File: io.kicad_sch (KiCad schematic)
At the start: 1 part, among them U1 Allwinner_V3s

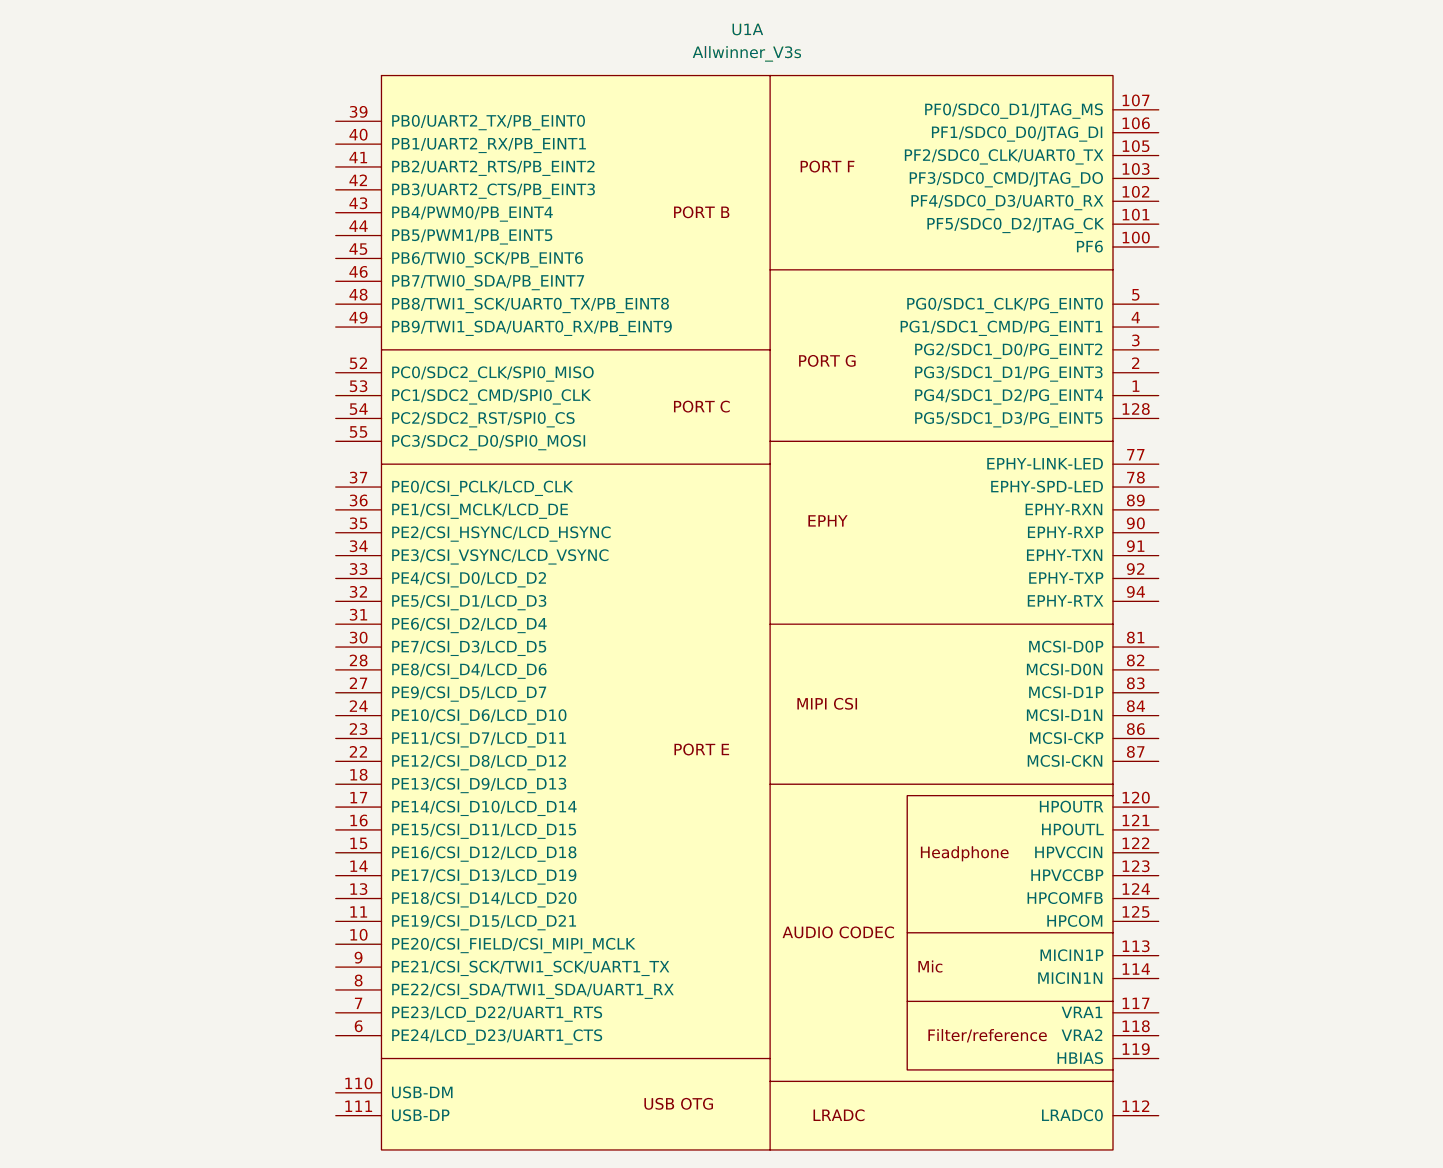
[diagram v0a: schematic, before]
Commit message: did some routing
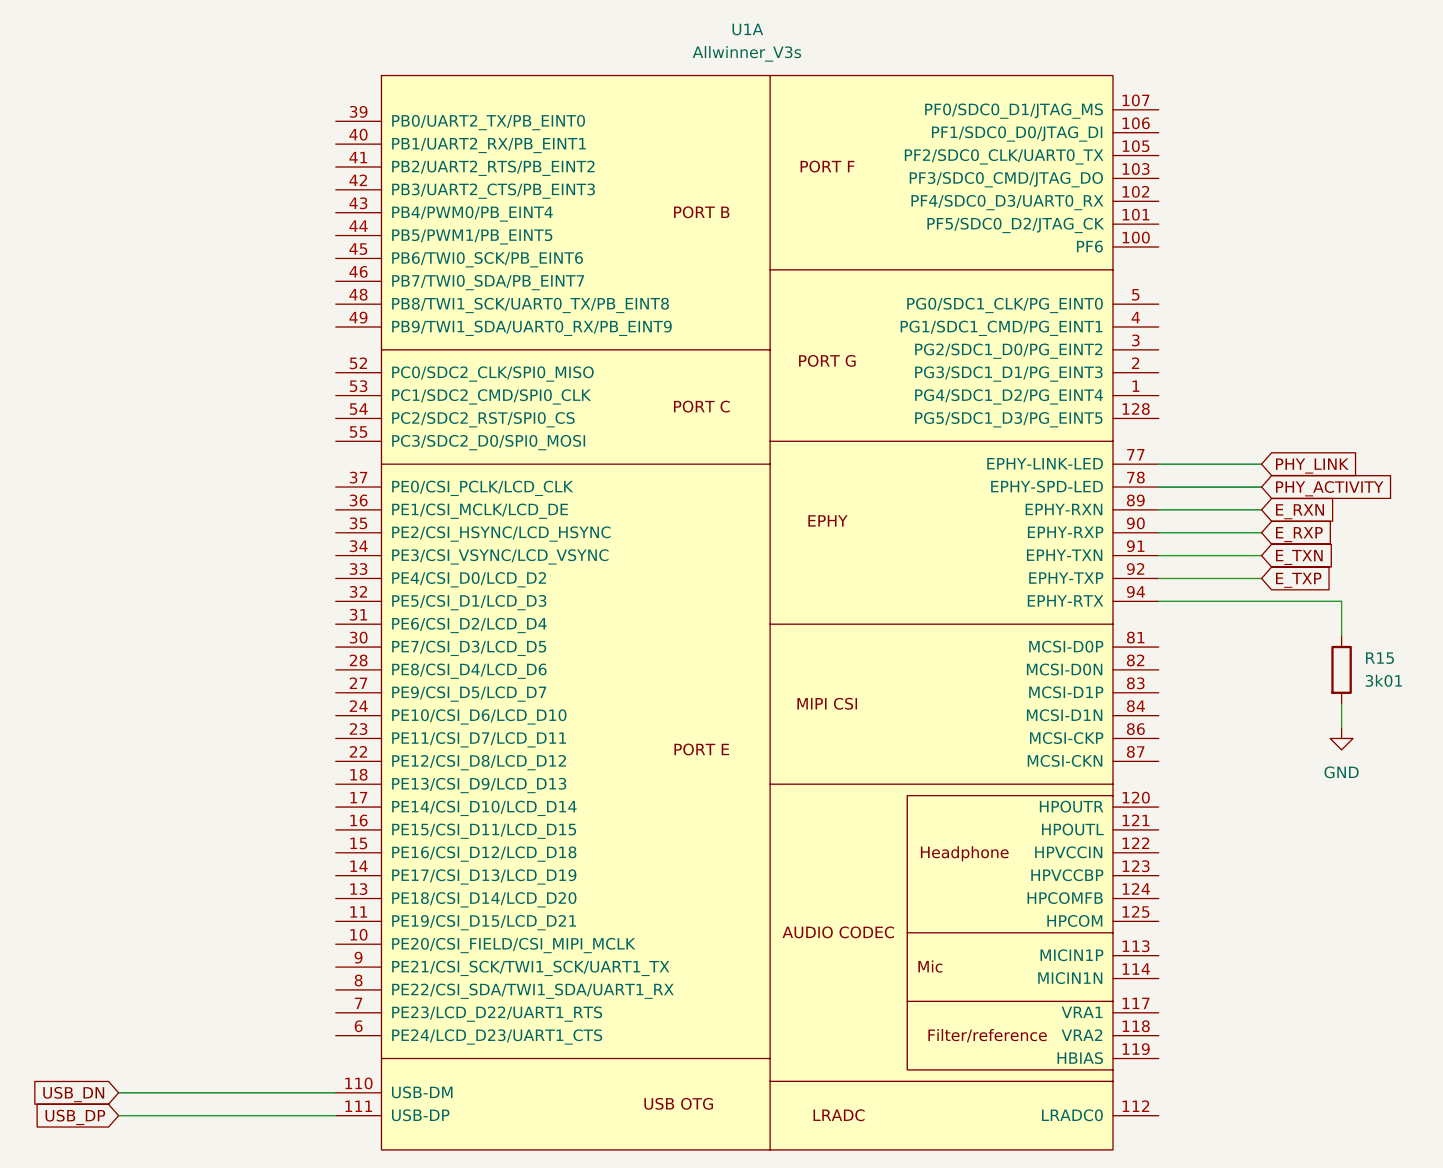
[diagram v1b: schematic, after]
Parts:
- added R15: 3k01, Resistor_SMD:R_0603_1608Metric, symbol Device:R
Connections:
- net USB_DN: now reaches U1.110 (USB-DM)
- net USB_DP: now reaches U1.111 (USB-DP)
- net PHY_LINK: now reaches U1.77 (EPHY-LINK-LED)
- net PHY_ACTIVITY: now reaches U1.78 (EPHY-SPD-LED)
- net E_RXN: now reaches U1.89 (EPHY-RXN)
- net E_RXP: now reaches U1.90 (EPHY-RXP)
- net E_TXN: now reaches U1.91 (EPHY-TXN)
- net E_TXP: now reaches U1.92 (EPHY-TXP)
- net at U1.94 (EPHY-RTX): now also R15.1
- new net GND: R15.2

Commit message: Updated BOM
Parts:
- R15: LCSC Part # (none) -> C22991
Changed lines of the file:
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@@
+			)
+		)
+		(property "LCSC Part #" ""
+			(at 143.51 95.25 0)
+			(hide yes)
+			(show_name no)
+			(do_not_autoplace no)
+			(effects
+				(font
+					(size 1.27 1.27)
+				)
+			)
+		)
+		(property "KLC_S3.3" ""
+			(at 143.51 95.25 0)
+			(hide yes)
+			(show_name no)
+			(do_not_autoplace no)
+			(effects
+				(font
+					(size 1.27 1.27)
+				)
+			)
+		)
+		(property "KLC_S4.1" ""
+			(at 143.51 95.25 0)
+			(hide yes)
+			(show_name no)
+			(do_not_autoplace no)
+			(effects
+				(font
+					(size 1.27 1.27)
+				)
+			)
+		)
+		(property "KLC_S4.2_DVDD" ""
+			(at 143.51 95.25 0)
+			(hide yes)
+			(show_name no)
+			(do_not_autoplace no)
+			(effects
+				(font
+					(size 1.27 1.27)
+				)
+			)
+		)
+		(property "KLC_S4.2_VREG_VOUT" ""
+			(at 143.51 95.25 0)
+			(hide yes)
+			(show_name no)
+			(do_not_autoplace no)
+			(effects
+				(font
+					(size 1.27 1.27)
+				)
 			)
 		)
@@
 			(at 207.01 100.33 0)
 			(hide yes)
+			(show_name no)
+			(do_not_autoplace no)
+			(effects
+				(font
+					(size 1.27 1.27)
+				)
+			)
+		)
+		(property "LCSC Part #" "C22991"
+			(at 207.01 100.33 0)
+			(hide yes)
+			(show_name no)
+			(do_not_autoplace no)
+			(effects
+				(font
+					(size 1.27 1.27)
+				)
+			)
+		)
+		(property "KLC_S3.3" ""
+			(at 207.01 100.33 0)
+			(hide yes)
+			(show_name no)
+			(do_not_autoplace no)
+			(effects
+				(font
+					(size 1.27 1.27)
+				)
+			)
+		)
+		(property "KLC_S4.1" ""
+			(at 207.01 100.33 0)
+			(hide yes)
+			(show_name no)
+			(do_not_autoplace no)
+			(effects
+				(font
+					(size 1.27 1.27)
+				)
+			)
+		)
+		(property "KLC_S4.2_DVDD" ""
+			(at 207.01 100.33 0)
+			(hide yes)
+			(show_name no)
+			(do_not_autoplace no)
+			(effects
+				(font
+					(size 1.27 1.27)
+				)
+			)
+		)
+		(property "KLC_S4.2_VREG_VOUT" ""
+			(at 207.01 100.33 0)
+			(hide yes)
